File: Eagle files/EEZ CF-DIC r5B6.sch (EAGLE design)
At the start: 275 parts, among them IC1 VIPer35L, IC2 SI8233BB-D-IS1, IC3 LM5041B, IC4 LM258D, IC5 IR11688STRPBF, IC6 LM258D, IC7 TL103W, P1 T910W-50K, Q1 MMBT5551, Q10 BC856C, Q2 C3M0280090D, Q3 C3M0280090D, Q4 NYC0102BLT1G, Q5 IPW60R125P6XKSA1, Q6 IPW60R125P6XKSA1, Q7 FDD86250-F085, Q8 FDD86250-F085, Q9 BC856C, X1 39-30-3035, X2 22-05-7085, X3 B2B-ZR, X4 39-30-1020

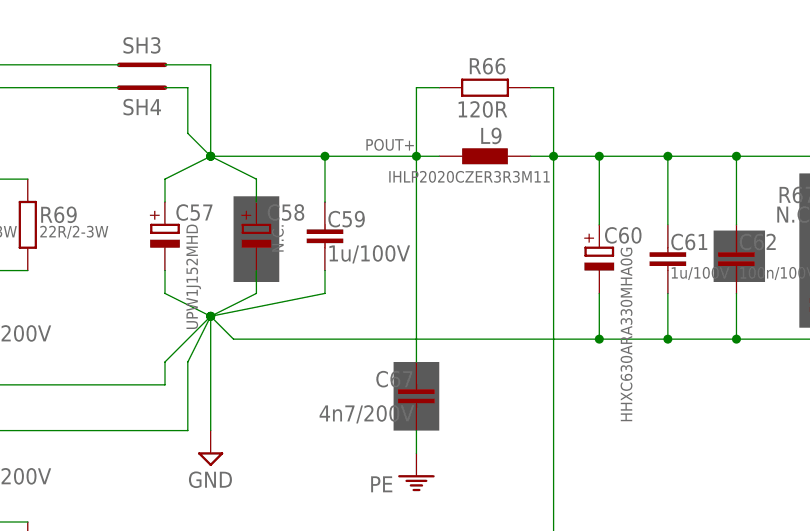
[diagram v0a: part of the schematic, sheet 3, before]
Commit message: BOM update
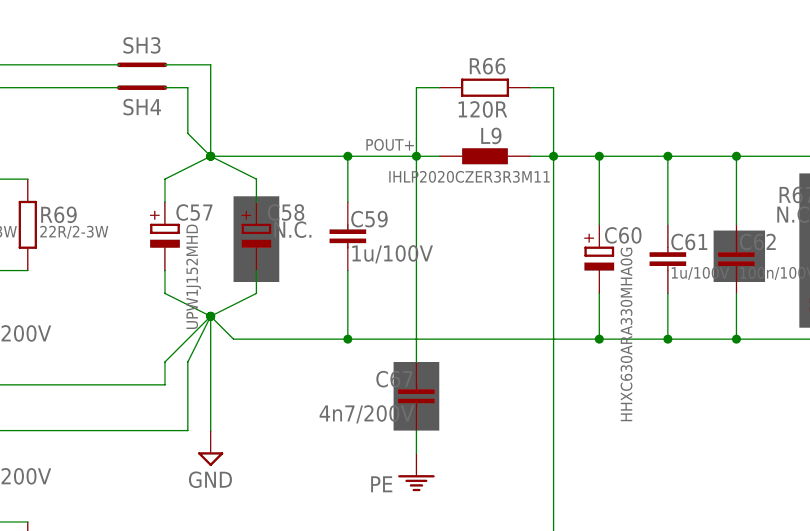
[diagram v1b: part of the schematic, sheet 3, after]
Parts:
- D10, D16, D19: device EEZ_Lib1:SCHOTTKY-SIC -> EEZ_Lib1:SCHOTTKY-SIC_L
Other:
- note added: "? IGBT: STGW10M65DF2 or FGH20N60UFDTU, Rg down to 10R ?"
- note removed: "86K6?"
- note removed: "IGBT: FGH20N60UFDTU"
- note removed: "IGBT: None"
- note removed: "IGBT: STGW10M65DF2"
- moved on the sheet: C59
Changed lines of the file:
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@@
 <setting verticaltext="up"/>
 </settings>
-<grid distance="0.025" unitdist="inch" unit="inch" style="lines" multiple="4" display="no" altdistance="0.01" altunitdist="inch" altunit="inch"/>
+<grid distance="0.1" unitdist="inch" unit="inch" style="lines" multiple="1" display="no" altdistance="0.01" altunitdist="inch" altunit="inch"/>
 <layers>
 <layer number="1" name="Top" color="4" fill="1" visible="no" active="no"/>
@@
 <part name="C37" library="rcl" deviceset="C-EU" device="C0603" value="100n"/>
 <part name="R52" library="rcl" deviceset="R-EU_" device="R0805" value="86K6"/>
-<part name="D10" library="EEZ_Lib1" deviceset="SCHOTTKY" device="-SIC" value="C3D02065E"/>
+<part name="D10" library="EEZ_Lib1" deviceset="SCHOTTKY" device="-SIC_L" value="C3D02065E"/>
 <part name="C31" library="rcl" deviceset="C-EU" device="C0603" value="10n"/>
 <part name="Q6" library="EEZ_Lib1" deviceset="IRFP240" device="" value="IPW60R125P6XKSA1"/>
@@
 <part name="R22" library="rcl" deviceset="R-EU_" device="R1206" value="100K"/>
 <part name="C44" library="rcl" deviceset="C-EU" device="C0805" value="1u"/>
-<part name="D16" library="EEZ_Lib1" deviceset="SCHOTTKY" device="-SIC" value="C3D02065E"/>
-<part name="D19" library="EEZ_Lib1" deviceset="SCHOTTKY" device="-SIC" value="C3D02065E"/>
+<part name="D16" library="EEZ_Lib1" deviceset="SCHOTTKY" device="-SIC_L" value="C3D02065E"/>
+<part name="D19" library="EEZ_Lib1" deviceset="SCHOTTKY" device="-SIC_L" value="C3D02065E"/>
 <part name="R42" library="rcl" deviceset="R-EU_" device="R2512" value="22R/2-3W"/>
 <part name="R23" library="rcl" deviceset="R-EU_" device="R0805" value="10R"/>
@@
 <rectangle x1="199.39" y1="63.5" x2="207.645" y2="67.945" layer="97"/>
 <text x="143.51" y="57.15" size="1.27" layer="100">Rct</text>
-<text x="55.88" y="74.295" size="1.27" layer="100">86K6?</text>
-<text x="170.18" y="151.13" size="1.27" layer="100">IGBT: STGW10M65DF2</text>
-<text x="157.48" y="125.095" size="1.27" layer="100">IGBT: None</text>
+<text x="232.41" y="74.93" size="1.27" layer="100">? IGBT: STGW10M65DF2 or
+FGH20N60UFDTU,
+Rg down to 10R ?</text>
 </plain>
 <instances>
@@
 <segment>
 <pinref part="D10" gate="G$1" pin="C"/>
-<wire x1="127" y1="167.64" x2="137.16" y2="167.64" width="0.1524" layer="91"/>
 <pinref part="IC2" gate="G$1" pin="VDDA"/>
 <pinref part="C31" gate="G$1" pin="1"/>
+<wire x1="127" y1="167.64" x2="137.16" y2="167.64" width="0.1524" layer="91"/>
 <wire x1="129.54" y1="149.86" x2="137.16" y2="149.86" width="0.1524" layer="91"/>
 <pinref part="C32" gate="G$1" pin="1"/>
@@
 <text x="5.08" y="40.005" size="1.778" layer="97">Active Duty cycle limiter</text>
 <wire x1="83.82" y1="10.16" x2="83.82" y2="43.18" width="0.1524" layer="97" style="shortdash"/>
-<text x="97.79" y="148.59" size="1.27" layer="100">IGBT: FGH20N60UFDTU</text>
-<text x="97.79" y="118.11" size="1.27" layer="100">IGBT: FGH20N60UFDTU</text>
 </plain>
 <instances>
@@
 <attribute name="VALUE" x="25.4" y="140.843" size="1.778" layer="96"/>
 </instance>
-<instance part="C59" gate="G$1" x="162.56" y="154.94" smashed="yes">
-<attribute name="NAME" x="162.814" y="154.686" size="1.778" layer="95"/>
-<attribute name="VALUE" x="162.814" y="150.876" size="1.778" layer="96"/>
+<instance part="C59" gate="G$1" x="165.1" y="154.94" smashed="yes">
+<attribute name="NAME" x="165.354" y="154.686" size="1.778" layer="95"/>
+<attribute name="VALUE" x="165.354" y="150.876" size="1.778" layer="96"/>
 </instance>
 <instance part="C66" gate="G$1" x="40.64" y="137.16" smashed="yes">
@@
 <instance part="C58" gate="G$1" x="154.94" y="154.94" smashed="yes">
 <attribute name="NAME" x="156.083" y="155.4226" size="1.778" layer="95"/>
-<attribute name="VALUE" x="156.6926" y="155.067" size="1.27" layer="96" rot="R270"/>
+<attribute name="VALUE" x="156.718" y="153.5176" size="1.778" layer="96"/>
 </instance>
 <instance part="D26" gate="G$1" x="91.44" y="160.02" smashed="yes" rot="R180">
@@
 <label x="248.92" y="142.875" size="1.27" layer="102" rot="MR0"/>
 <pinref part="C59" gate="G$1" pin="2"/>
-<wire x1="162.56" y1="149.86" x2="162.56" y2="147.32" width="0.1524" layer="91"/>
-<wire x1="162.56" y1="147.32" x2="149.86" y2="144.78" width="0.1524" layer="91"/>
 <junction x="149.86" y="144.78"/>
 <pinref part="C63" gate="G$1" pin="2"/>
@@
 <pinref part="C57" gate="G$1" pin="-"/>
 <pinref part="C58" gate="G$1" pin="-"/>
-<wire x1="193.04" y1="142.24" x2="152.4" y2="142.24" width="0.1524" layer="91"/>
+<wire x1="193.04" y1="142.24" x2="165.1" y2="142.24" width="0.1524" layer="91"/>
+<wire x1="165.1" y1="142.24" x2="152.4" y2="142.24" width="0.1524" layer="91"/>
 <wire x1="154.94" y1="149.86" x2="154.94" y2="147.32" width="0.1524" layer="91"/>
 <wire x1="154.94" y1="147.32" x2="149.86" y2="144.78" width="0.1524" layer="91"/>
@@
 <wire x1="208.28" y1="147.32" x2="208.28" y2="142.24" width="0.1524" layer="91"/>
 <junction x="208.28" y="142.24"/>
+<wire x1="165.1" y1="149.86" x2="165.1" y2="142.24" width="0.1524" layer="91"/>
+<junction x="165.1" y="142.24"/>
 </segment>
 <segment>
@@
 <segment>
 <pinref part="C59" gate="G$1" pin="1"/>
-<wire x1="162.56" y1="162.56" x2="172.72" y2="162.56" width="0.1524" layer="91"/>
-<wire x1="162.56" y1="157.48" x2="162.56" y2="162.56" width="0.1524" layer="91"/>
-<junction x="162.56" y="162.56"/>
+<wire x1="165.1" y1="162.56" x2="172.72" y2="162.56" width="0.1524" layer="91"/>
+<wire x1="165.1" y1="157.48" x2="165.1" y2="162.56" width="0.1524" layer="91"/>
+<junction x="165.1" y="162.56"/>
 <junction x="149.86" y="162.56"/>
 <wire x1="144.78" y1="170.18" x2="147.32" y2="170.18" width="0.1524" layer="91"/>
@@
 <wire x1="149.86" y1="162.56" x2="149.86" y2="172.72" width="0.1524" layer="91"/>
 <wire x1="149.86" y1="172.72" x2="144.78" y2="172.72" width="0.1524" layer="91"/>
-<wire x1="149.86" y1="162.56" x2="162.56" y2="162.56" width="0.1524" layer="91"/>
+<wire x1="149.86" y1="162.56" x2="165.1" y2="162.56" width="0.1524" layer="91"/>
 <pinref part="C58" gate="G$1" pin="+"/>
-<wire x1="154.94" y1="160.02" x2="154.94" y2="157.48" width="0.1524" layer="91"/>
 <wire x1="149.86" y1="162.56" x2="154.94" y2="160.02" width="0.1524" layer="91"/>
+<wire x1="154.94" y1="160.02" x2="154.94" y2="157.48" width="0.1524" layer="91"/>
 <pinref part="C57" gate="G$1" pin="+"/>
 <wire x1="144.78" y1="157.48" x2="144.78" y2="160.02" width="0.1524" layer="91"/>
